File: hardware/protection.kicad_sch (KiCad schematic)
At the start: 4 parts

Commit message: kończymy balet na dziś
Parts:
- C5: footprint Capacitor_SMD:C_0201_0603Metric_Pad0.64x0.40mm_HandSolder -> Capacitor_SMD:C_0603_1608Metric_Pad1.08x0.95mm_HandSolder
- R10, R11: footprint Resistor_SMD:R_0603_1608Metric -> Resistor_SMD:R_0603_1608Metric_Pad0.98x0.95mm_HandSolder
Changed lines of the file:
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@@
       (effects (font (size 1.27 1.27)) (justify left))
     )
-    (property "Footprint" "Capacitor_SMD:C_0201_0603Metric_Pad0.64x0.40mm_HandSolder" (id 2) (at 119.0752 49.53 0)
+    (property "Footprint" "Capacitor_SMD:C_0603_1608Metric_Pad1.08x0.95mm_HandSolder" (id 2) (at 119.0752 49.53 0)
       (effects (font (size 1.27 1.27)) hide)
     )
@@
       (effects (font (size 1.27 1.27)) (justify left))
     )
-    (property "Footprint" "Resistor_SMD:R_0603_1608Metric" (id 2) (at 78.232 34.29 90)
+    (property "Footprint" "Resistor_SMD:R_0603_1608Metric_Pad0.98x0.95mm_HandSolder" (id 2) (at 78.232 34.29 90)
       (effects (font (size 1.27 1.27)) hide)
     )
@@
       (effects (font (size 1.27 1.27)) (justify left))
     )
-    (property "Footprint" "Resistor_SMD:R_0603_1608Metric" (id 2) (at 78.232 44.45 90)
+    (property "Footprint" "Resistor_SMD:R_0603_1608Metric_Pad0.98x0.95mm_HandSolder" (id 2) (at 78.232 44.45 90)
       (effects (font (size 1.27 1.27)) hide)
     )

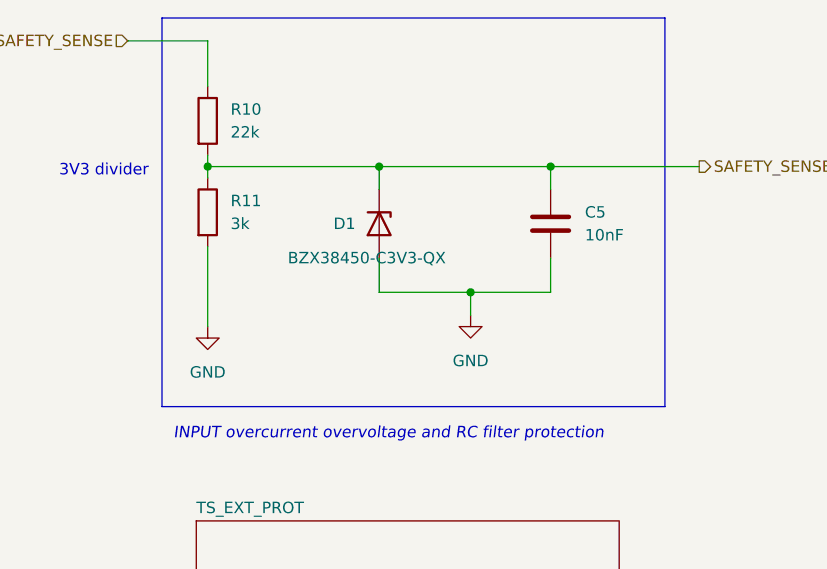
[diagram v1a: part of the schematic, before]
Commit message: uploaded older pcb version
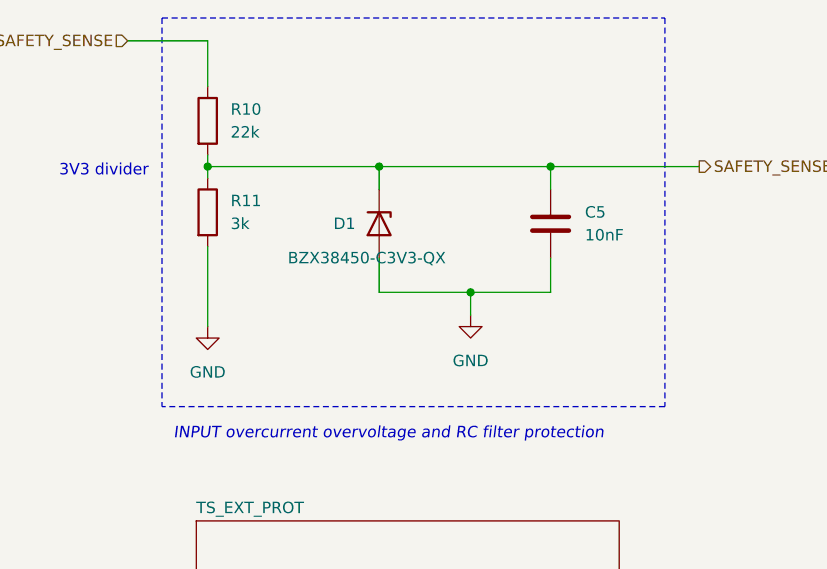
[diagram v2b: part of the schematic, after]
